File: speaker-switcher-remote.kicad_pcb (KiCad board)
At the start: 2 copper layers, 50 x 70 mm, 30 parts, among them M1 arduino-nano, Q1 2N2222, Q2 TIP31C, U1 LM7805_TO220

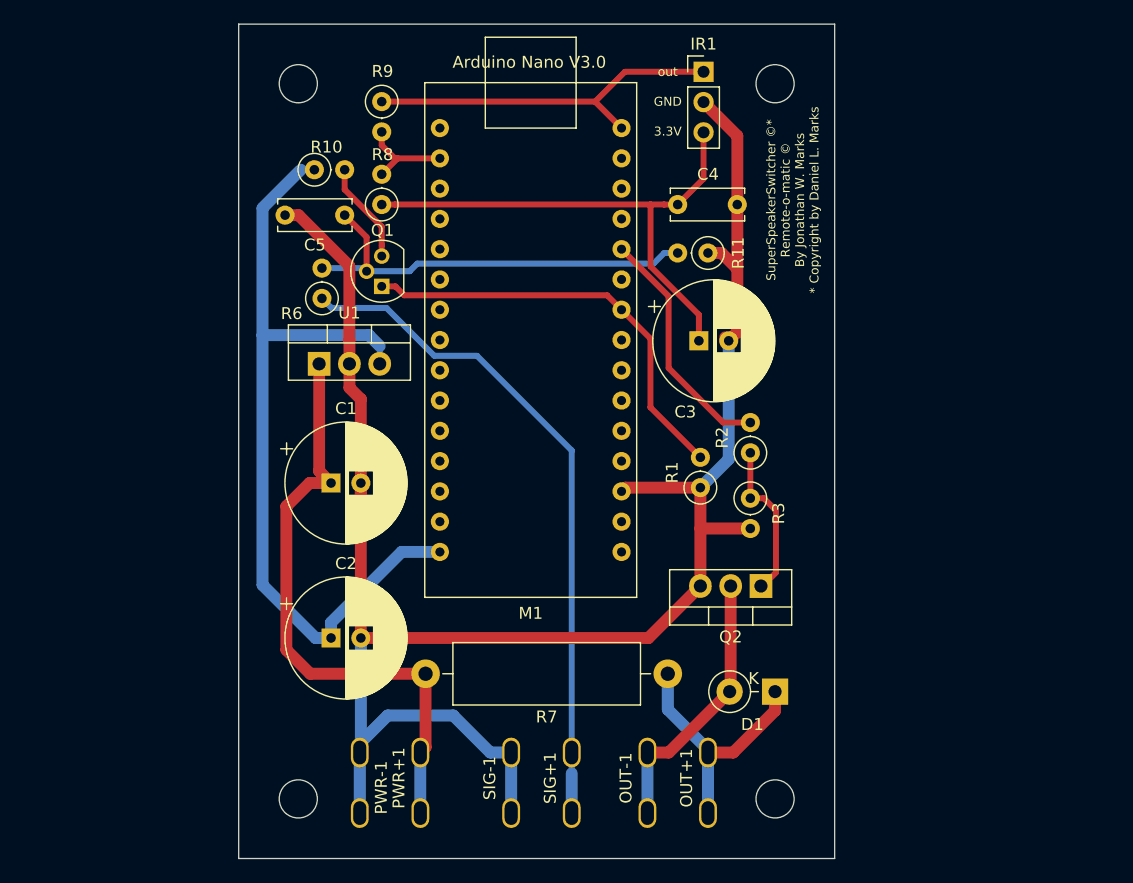
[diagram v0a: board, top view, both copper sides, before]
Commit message: Updated PCB but not plots
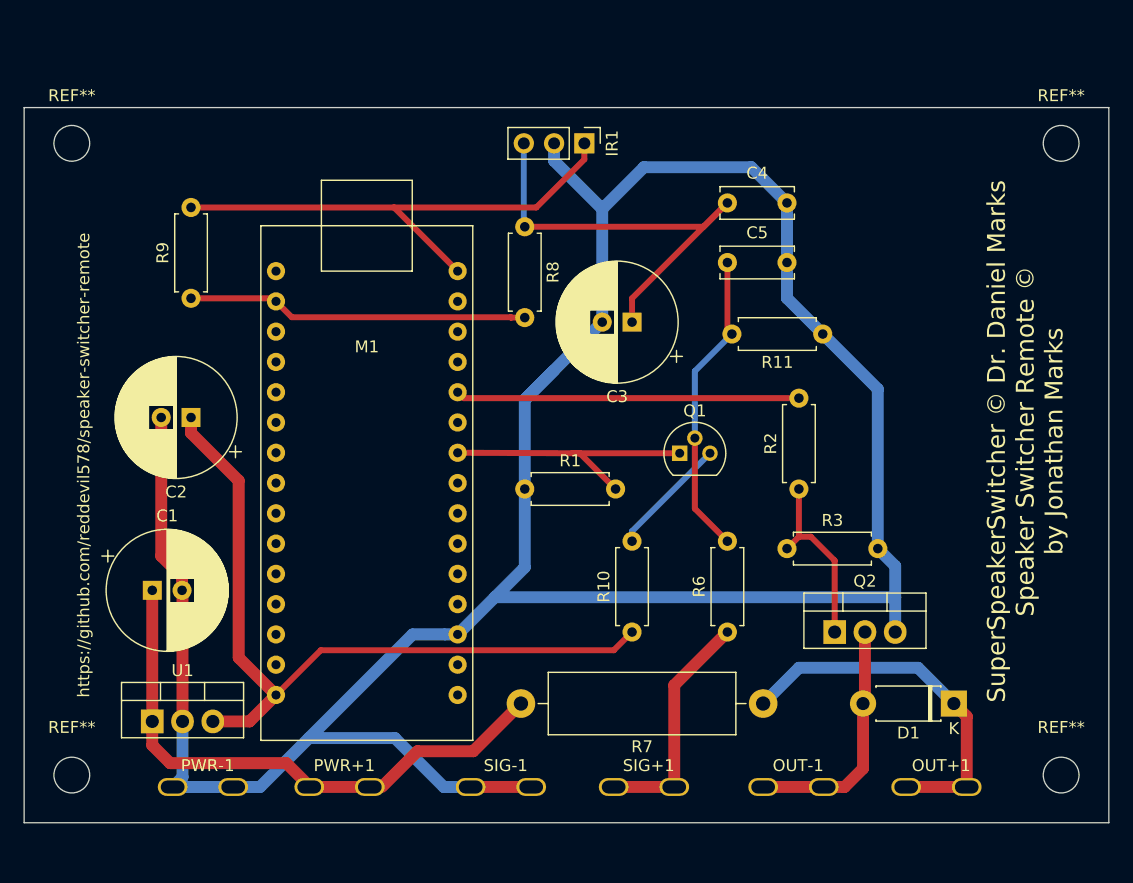
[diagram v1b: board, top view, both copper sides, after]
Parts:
- removed the REF** at (166.2, 126.5)
- removed the REF** at (126.2, 126.5)
- removed the REF** at (126.2, 66.5)
- removed the REF** at (166.2, 66.5)
- added REF**: MountingHole_3mm, MountingHole:MountingHole_3mm, F.Cu at (190.2, 71.5)
- added REF**: MountingHole_3mm, MountingHole:MountingHole_3mm, F.Cu at (107.2, 71.5)
- added REF**: MountingHole_3mm, MountingHole:MountingHole_3mm, F.Cu at (107.2, 124.5)
- added REF**: MountingHole_3mm, MountingHole:MountingHole_3mm, F.Cu at (190.2, 124.5)
- D1: footprint Diode_THT:D_DO-41_SOD81_P3.81mm_Vertical_KathodeUp -> Diode_THT:D_DO-41_SOD81_P7.62mm_Horizontal
- R1, R10, R11, R2, R3, R6, R8, R9: footprint Resistor_THT:R_Axial_DIN0207_L6.3mm_D2.5mm_P2.54mm_Vertical -> Resistor_THT:R_Axial_DIN0207_L6.3mm_D2.5mm_P7.62mm_Horizontal
- moved R10 47.1 mm to (154.2, 112.5), turned to 90 degrees
- moved R6 44.1 mm to (162.2, 112.5)
- moved U1 33.1 mm to (114.0, 120.0)
- moved C5 32.4 mm to (162.2, 81.5), turned to 0 degrees
- moved Q1 28.7 mm to (158.2, 97.5), turned to 0 degrees
- moved R9 23.0 mm to (117.2, 84.5), turned to 90 degrees
- moved C2 21.9 mm to (117.2, 94.5), turned to 180 degrees
- moved OUT+1 19.2 mm to (179.8, 125.5), turned to 0 degrees
- moved M1 18.2 mm to (132.0, 100.0)
- moved C1 17.5 mm to (114.0, 109.0)
- moved D1 15.0 mm to (181.2, 118.5)
- moved R1 14.7 mm to (145.2, 100.5), turned to 0 degrees
- moved PWR-1 13.2 mm to (118.2, 125.5), turned to 0 degrees
- moved OUT-1 12.3 mm to (167.8, 125.5), turned to 0 degrees
- moved R8 12.1 mm to (145.2, 78.5), turned to 270 degrees
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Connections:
- R9 pad 1: Net-(IR1-Pad1) -> Net-(M1-Pad2)
- R9 pad 2: Net-(M1-Pad2) -> Net-(IR1-Pad1)
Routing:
- net GNDREF: track 163.4 -> 224.9 mm
- net Net-(R6-Pad1): track 56.7 -> 19.9 mm
- net Net-(M1-Pad2): track 8.35 -> 28.7 mm
- net Net-(IR1-Pad1): track 31.2 -> 44.1 mm
- net Net-(M1-Pad22): track 36.1 -> 23.5 mm
- net Net-(C5-Pad1): track 36.1 -> 26.0 mm
- net Net-(D1-Pad1): track 21.7 -> 31.0 mm
- net Net-(M1-Pad20): track 20.4 -> 28.8 mm
- net Net-(C3-Pad1): track 44.9 -> 38.3 mm
- net +5V: track 69.5 -> 64.5 mm
- net PWR: track 51.4 -> 47.5 mm
- net Net-(D1-Pad2): track 23.0 -> 20.5 mm
- net Net-(Q2-Pad1): track 13.5 -> 15.2 mm
- net Net-(Q1-Pad3): track 9.32 -> 10.1 mm
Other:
- board size 50 x 70 mm -> 91 x 60 mm
- board text added: "SuperSpeakerSwitcher © Dr. Daniel Marks Speaker Switcher Remote © by Jonathan Marks"
- board text added: "https://github.com/reddevil578/speaker-switcher-remote"
- board text removed: "3.3V"
- board text removed: "Arduino Nano V3.0"
- board text removed: "GND"
- board text removed: "SuperSpeakerSwitcher ©* Remote-o-matic © By Jonathan W. Marks * Copyright by Daniel L. Marks"
- board text removed: "out"
